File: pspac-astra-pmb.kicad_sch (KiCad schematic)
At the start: 11 parts, among them J1 Conn_01x02_Socket, J2 Conn_01x01_Socket, J3 Screw_Terminal_01x03, J4 Screw_Terminal_01x02, Q1 BSC014N04LSIATMA1, U1 INA226

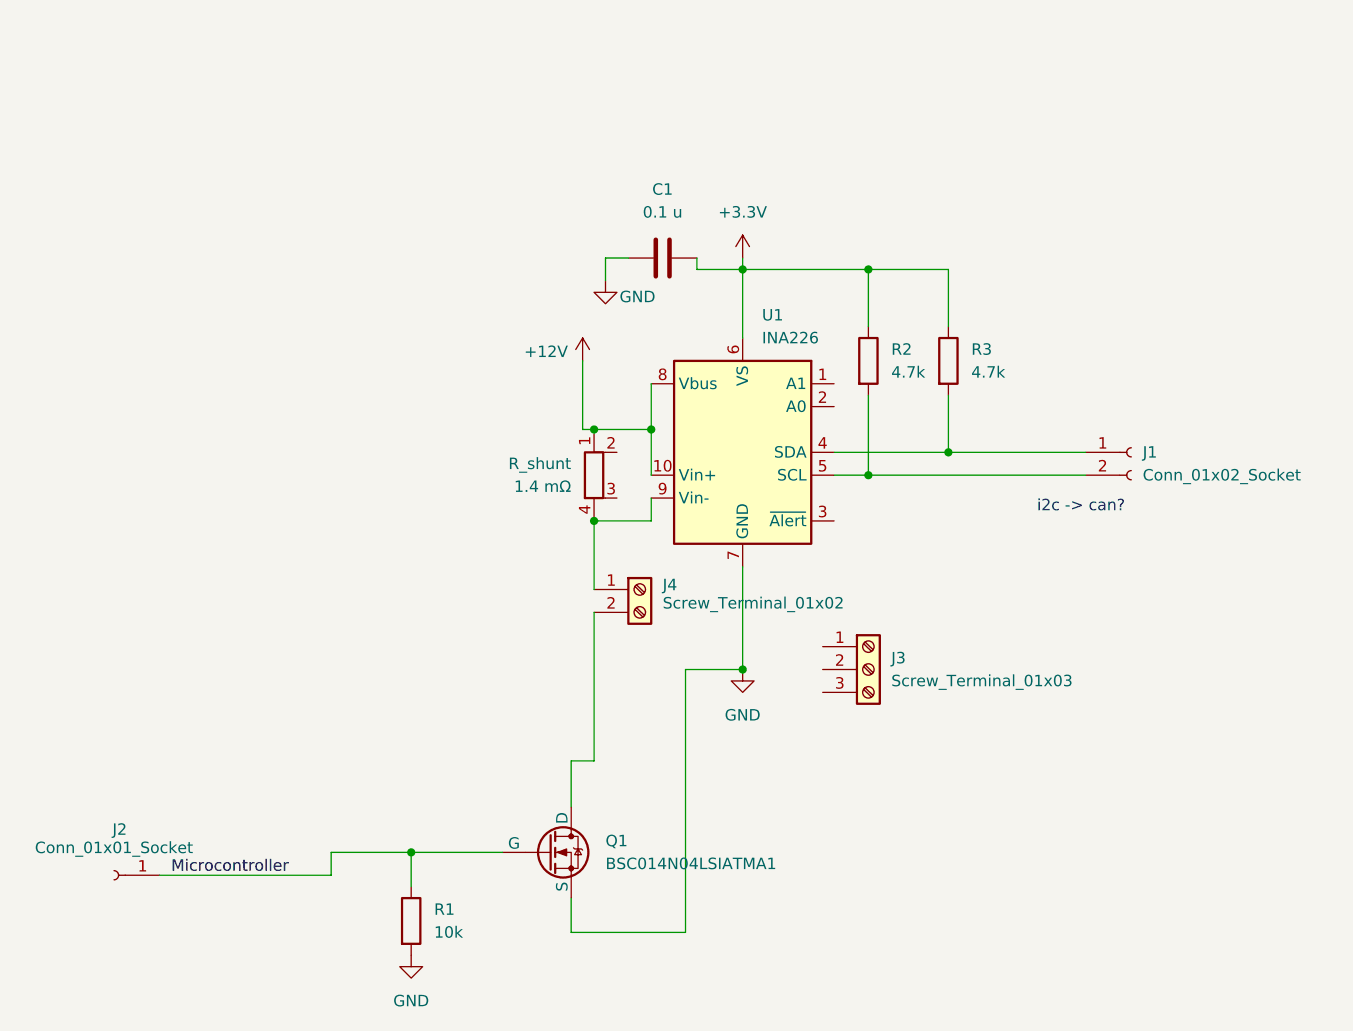
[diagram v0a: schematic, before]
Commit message: Add files via upload
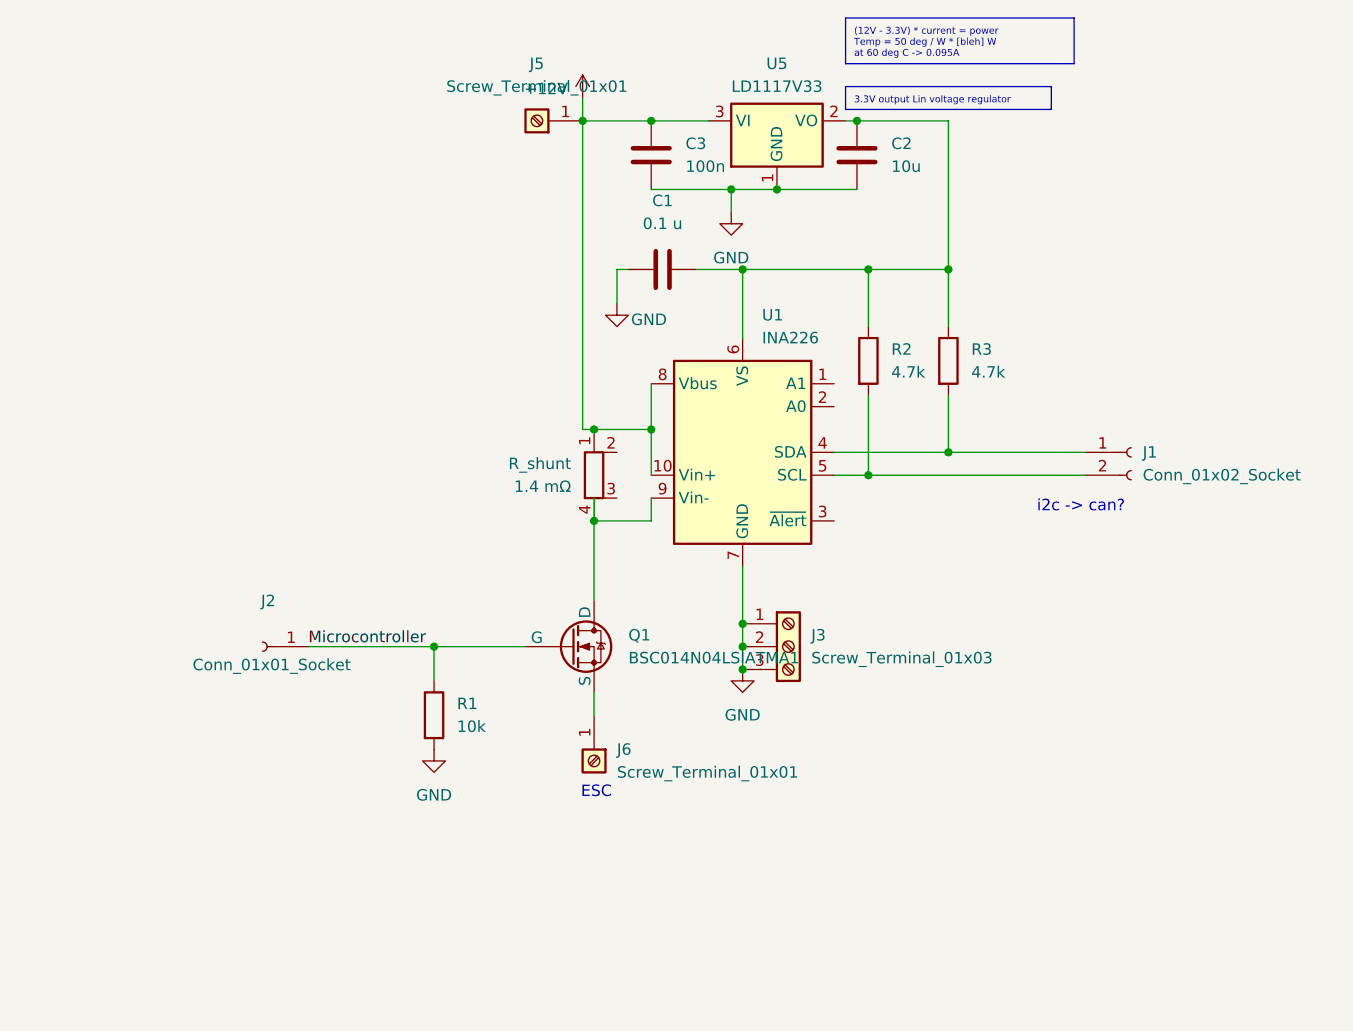
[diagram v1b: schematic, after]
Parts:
- removed J4: Screw_Terminal_01x02, TerminalBlock:TerminalBlock_bornier-2_P5.08mm, symbol Connector:Screw_Terminal_01x02
- added C2: 10u, symbol Device:C
- added C3: 100n, symbol Device:C
- added J5, J6: Screw_Terminal_01x01, symbol Connector:Screw_Terminal_01x01
- added U5: LD1117V33, Package_TO_SOT_THT:TO-220-3_Vertical, symbol Regulator_Linear:LD1117V33
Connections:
- net +12V: now also C3.1, J5.1 (Pin_1), U5.3 (VI)
- net GND: now also J3.1 (Pin_1), J3.2 (Pin_2), J3.3 (Pin_3), C2.2, C3.2, U5.1 (GND); no longer Q1.3 (S)
- net at R_shunt.4, U1.9 (Vin-): now also Q1.1 (D)
- net +3.3V: no longer names the net of C1.2, R2.1, R3.1, U1.6 (VS)
- net +3.3V: now also C2.1, U5.2 (VO)
- new net: J6.1 (Pin_1), Q1.3 (S)
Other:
- note added: "ESC"
- moved on the sheet: C1, J2, J3, Q1, R1
